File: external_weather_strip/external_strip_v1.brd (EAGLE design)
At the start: 100 x 80 mm, 10 parts, among them U1 ML8511-UV-SENSOR, U2 SHT21, U9 BMP180

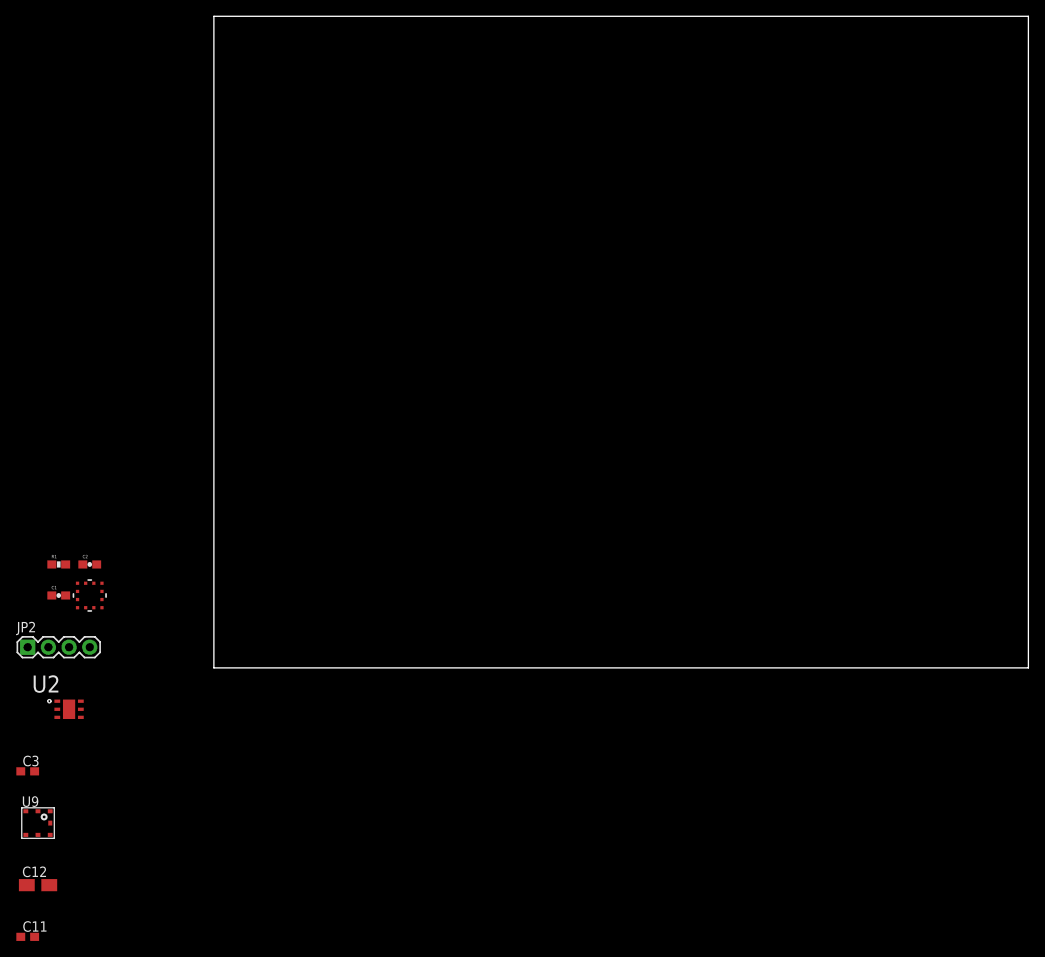
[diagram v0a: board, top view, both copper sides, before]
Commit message: layouting 0.4
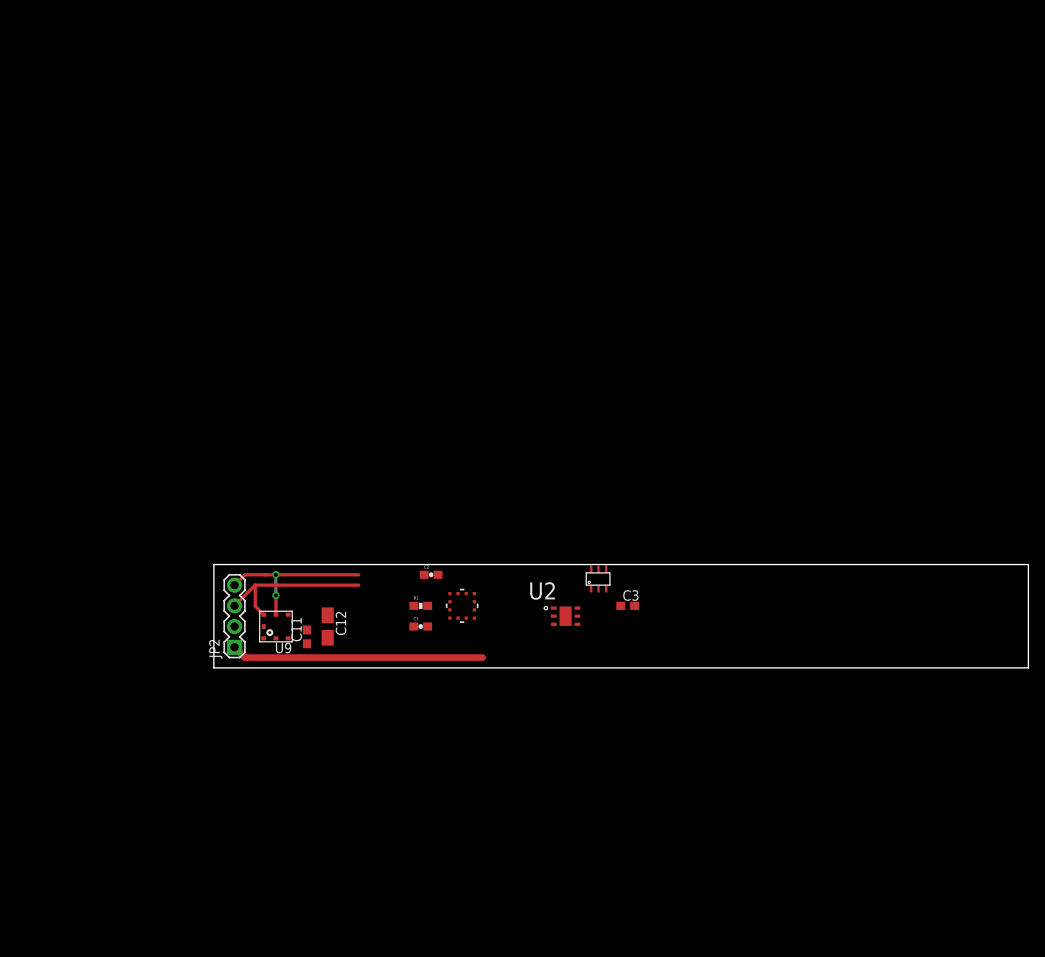
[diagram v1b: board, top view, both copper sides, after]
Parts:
- added U$5: MCP3425, phMeter:SOT-23-6
- moved C3 76.4 mm to (50.8, 7.62)
- moved U2 62.0 mm to (43.2, 6.35)
- moved C11 50.3 mm to (11.4, 3.81), turned to 90 degrees
- moved C12 47.7 mm to (14.0, 5.08), turned to 270 degrees
- moved U1 45.7 mm to (30.5, 7.62), turned to 90 degrees
- moved R1 44.7 mm to (25.4, 7.62)
- moved C1 44.6 mm to (25.4, 5.08)
- moved C2 41.9 mm to (26.7, 11.4)
- moved U9 37.9 mm to (7.62, 5.08), turned to 180 degrees
- moved JP2 25.4 mm to (2.54, 2.54), turned to 90 degrees
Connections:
- net ENABLE: no longer JP2.4
- net OUT: no longer JP2.3
- net SCL: now also JP2.4
- net SDA: now also JP2.3
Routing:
- net 3.3V: track 0.00 -> 31.0 mm
- net SCL: track 0.00 -> 20.7 mm, vias 0 -> 2
- net SDA: track 0.00 -> 20.4 mm
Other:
- board size 100 x 80 mm -> 100 x 12.7 mm

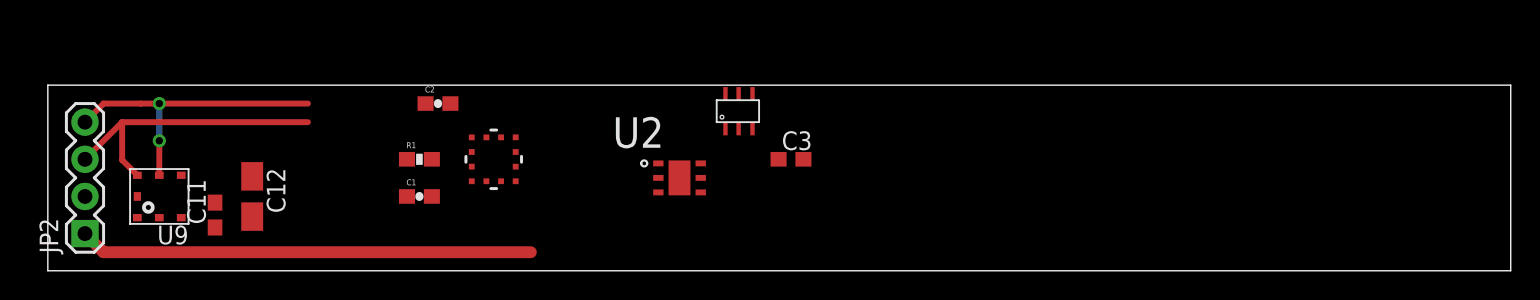
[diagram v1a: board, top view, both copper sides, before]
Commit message: finished weather strip
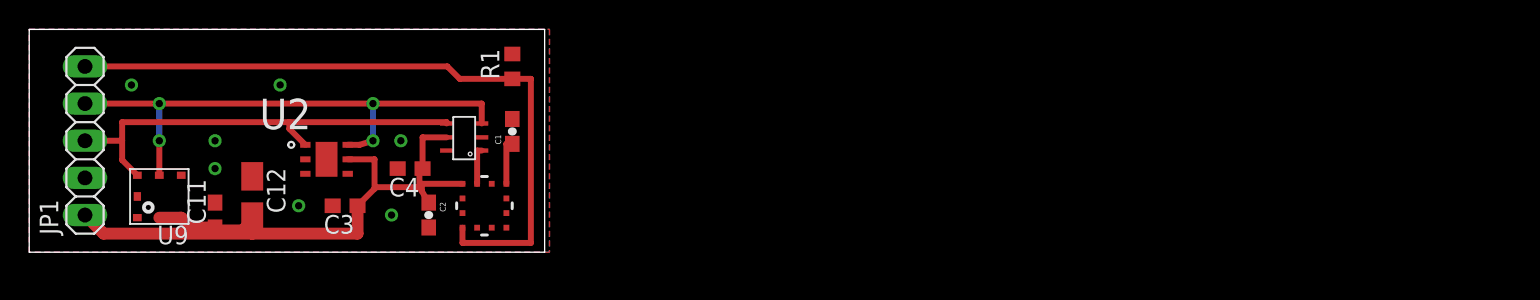
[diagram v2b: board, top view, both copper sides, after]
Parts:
- removed JP2: (no value), SparkFun-Connectors:1X04
- added C4: 100n, rcl:C0603
- added JP1: (no value), Headerlibrary:1X05
- R1: value 10K -> 10k; device SparkFun-Resistors:0603-RES -> resistor:R0603
- moved C3 30.6 mm to (20.3, 4.45), turned to 180 degrees
- moved U2 24.2 mm to (19.1, 7.62)
- moved U$5 16.7 mm to (29.2, 7.62), turned to 90 degrees
- moved R1 8.98 mm to (31.8, 14.0), turned to 90 degrees
- moved C1 7.75 mm to (31.8, 9.53), turned to 90 degrees
- moved C2 7.65 mm to (26.0, 3.81), turned to 270 degrees
- moved U1 3.24 mm to (29.8, 4.45)
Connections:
- removed net 3.3V: C2.1, JP2.1, R1.2, U1.7
- removed net ENABLE: R1.1, U1.4
- removed net OUT: U1.8
- new net N$1: U$5.VIN+, U1.8
- new net UV_EN: JP1.5, R1.1, U1.4
- net +3V3: now also C2.1, C4.1, JP1.1, U$5.VDD, U1.7
- net GND: now also C4.2, JP1.2, R1.2, U$5.VIN-, U$5.VSS; no longer JP2.2
- net SCL: now also JP1.4, U$5.SCL; no longer JP2.4
- net SDA: now also JP1.3, U$5.SDA; no longer JP2.3
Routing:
- net +3V3: track 0.00 -> 48.9 mm
- net UV_EN: track 0.00 -> 47.8 mm
- net 3.3V: track 31.0 -> 0.00 mm
- net SCL: track 20.7 -> 37.7 mm, vias 2 -> 4
- net SDA: track 20.4 -> 30.9 mm
- net N$3: track 0.00 -> 3.14 mm
- net N$1: track 0.00 -> 2.59 mm
- added copper zone on layer 1, net GND
- added copper zone on layer 16, net GND
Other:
- board size 100 x 12.7 mm -> 35.2 x 15.2 mm
- board text added: "3V3 GND SDA SCL UVEN"
- board text added: "MCP3425"
- board text added: "ML8511"
- board text added: "Octanis 1 weather monitor v1"
- board text added: "www.octanis.org"
